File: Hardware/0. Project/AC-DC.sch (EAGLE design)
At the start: 40 parts, among them IC1 LM358N, IC3 7812TV, K1 APF30212C, Q1 BC548B, Q2 BC558B, Q3 BC558B, SW1 CT10-XXXX-A2, U1 LM338K

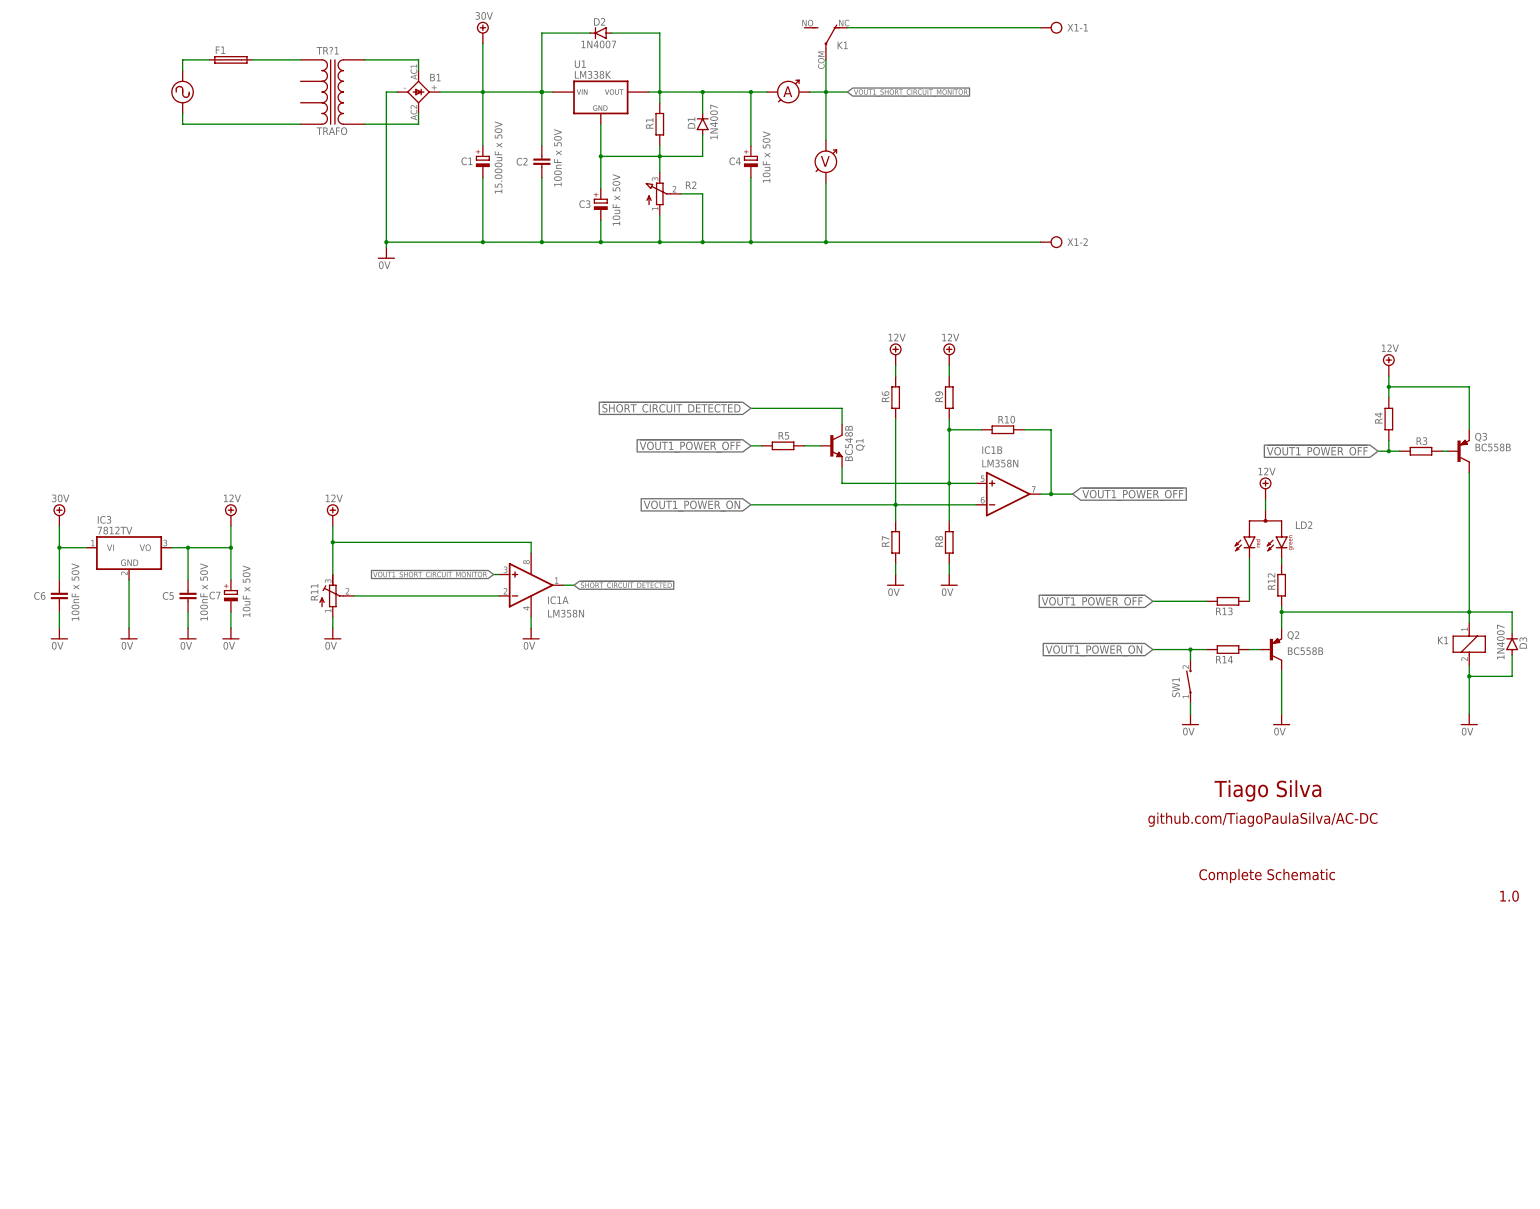
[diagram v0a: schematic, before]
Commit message: sch
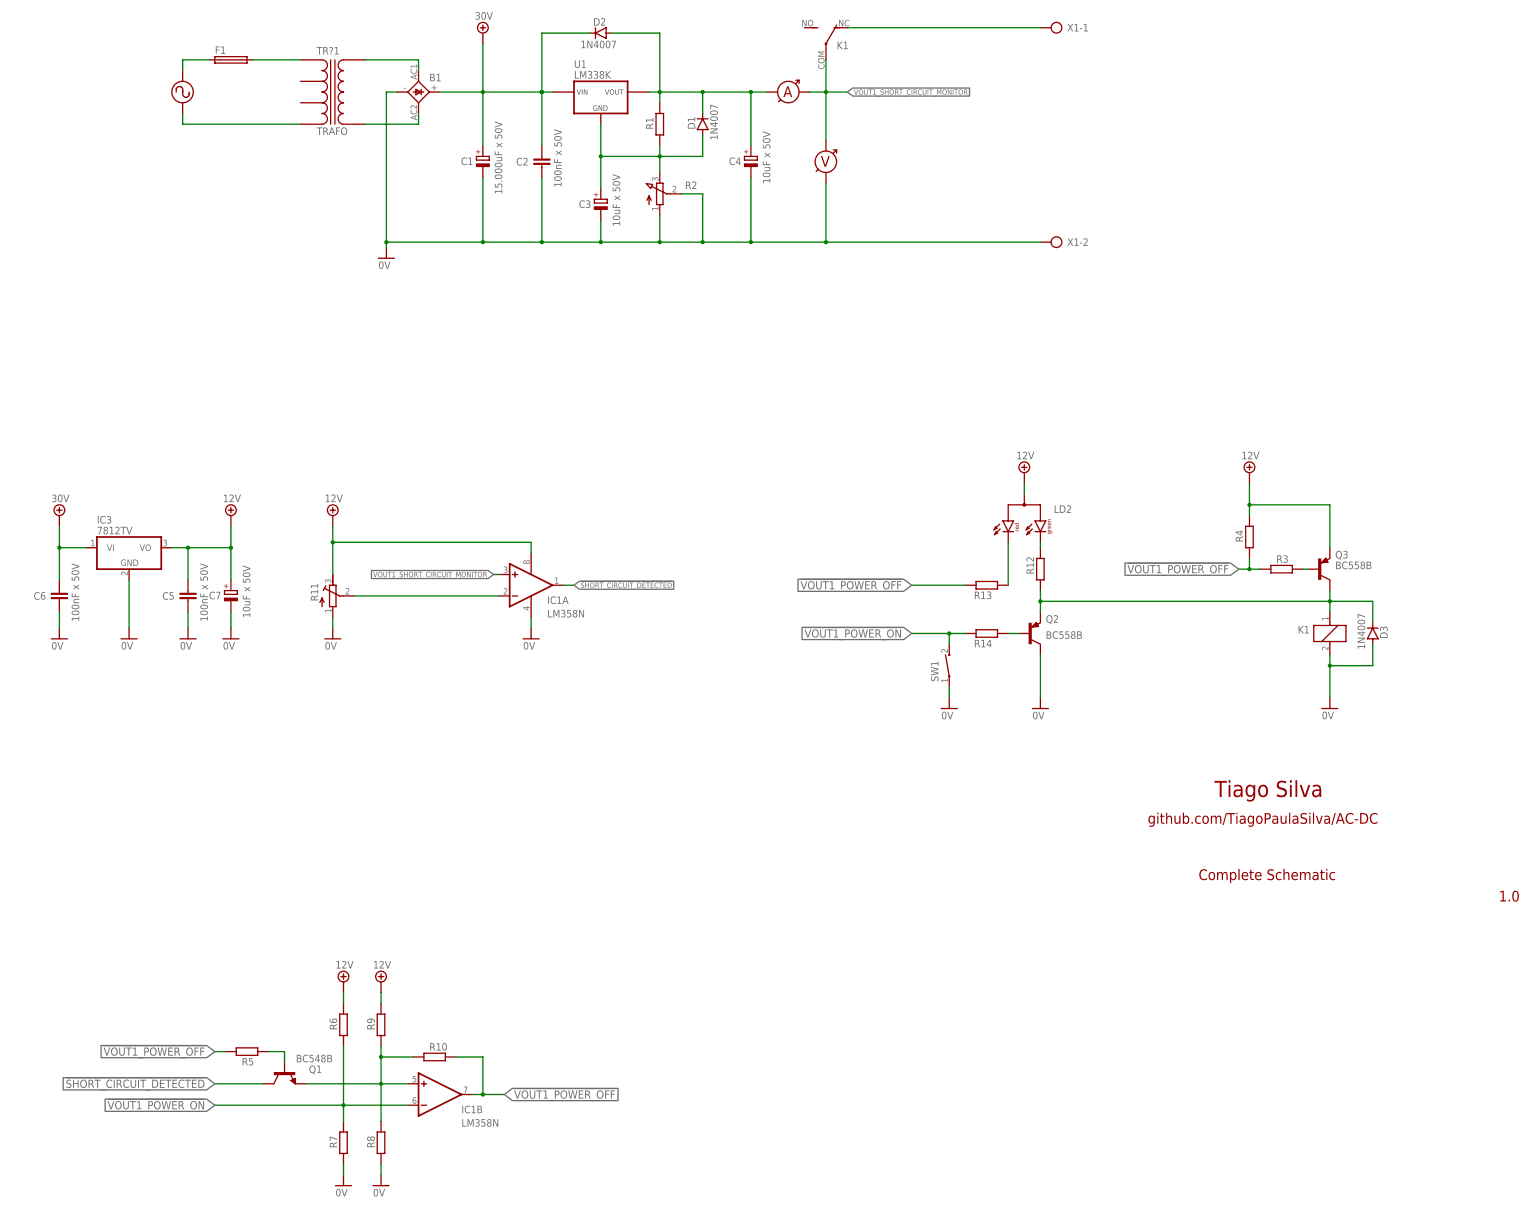
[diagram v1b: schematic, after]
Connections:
- net VOUT1_POWER_ON renamed !VOUT1_POWER_ON!
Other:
- moved on the sheet: D3, IC1B, K1, LD2, Q1, Q2, Q3, R10, R12, R13, R14, R3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
